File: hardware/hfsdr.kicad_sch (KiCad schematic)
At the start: 56 parts, among them J1 USB_C_Receptacle_USB2.0_16P, SW1 RST, SW2 BOOT0, SW4 EC12E2430803, U3 CH32V30xRxTx

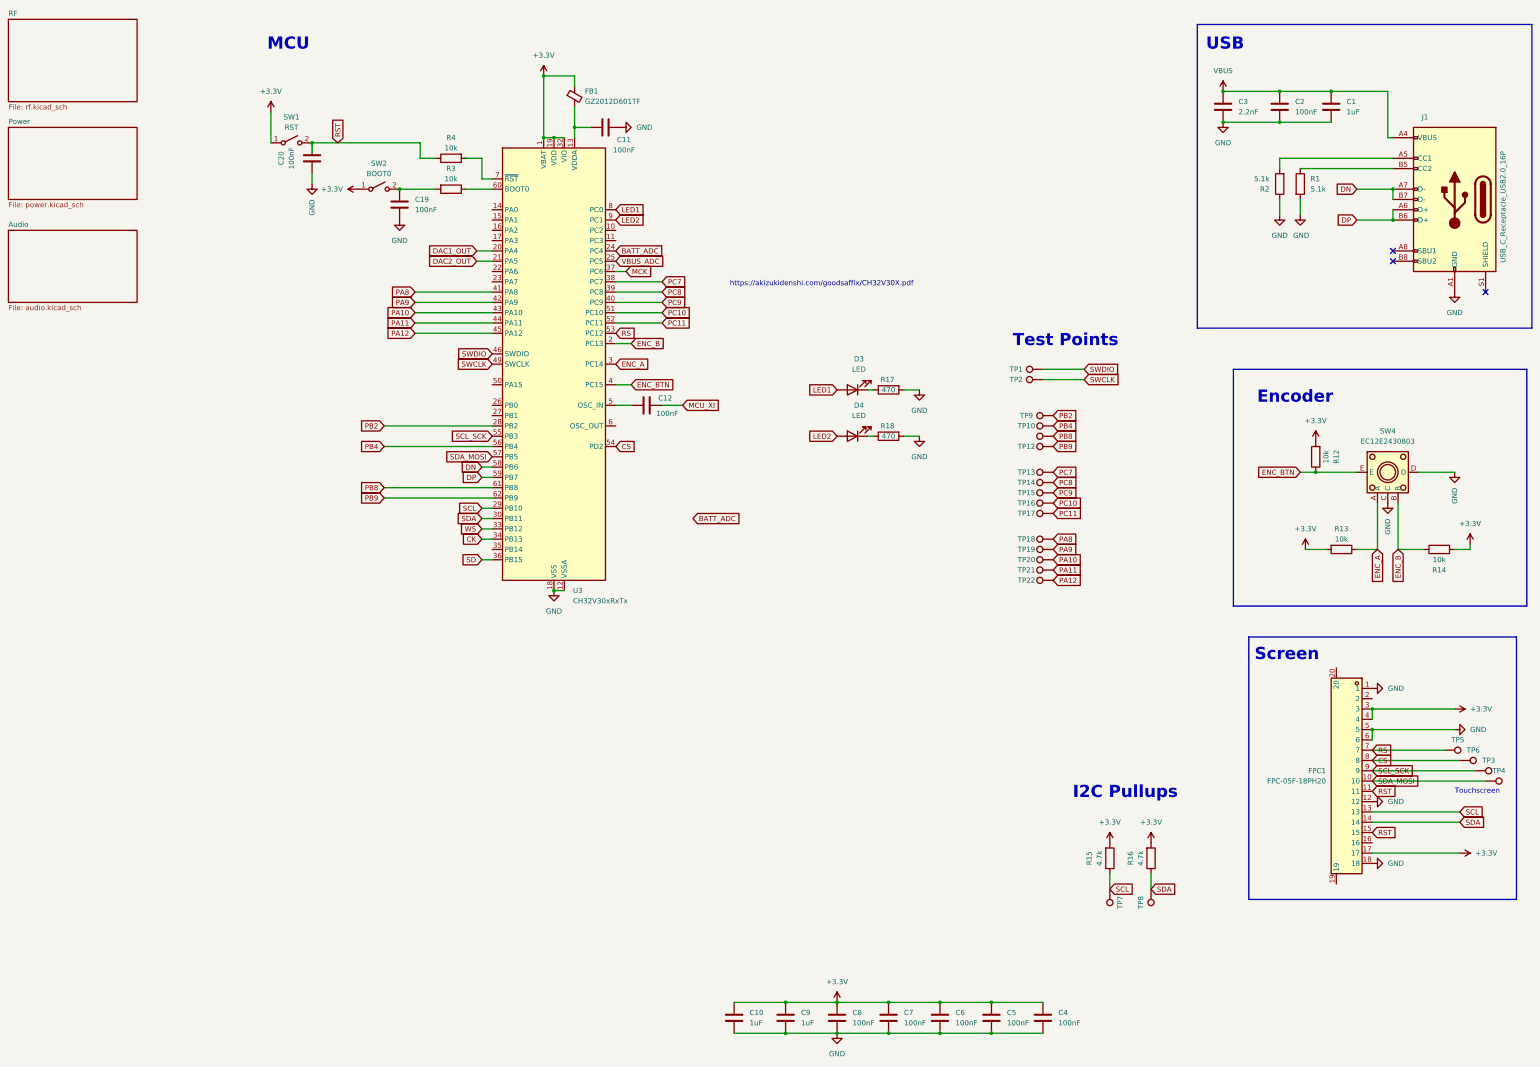
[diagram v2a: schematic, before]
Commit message: Update hardware
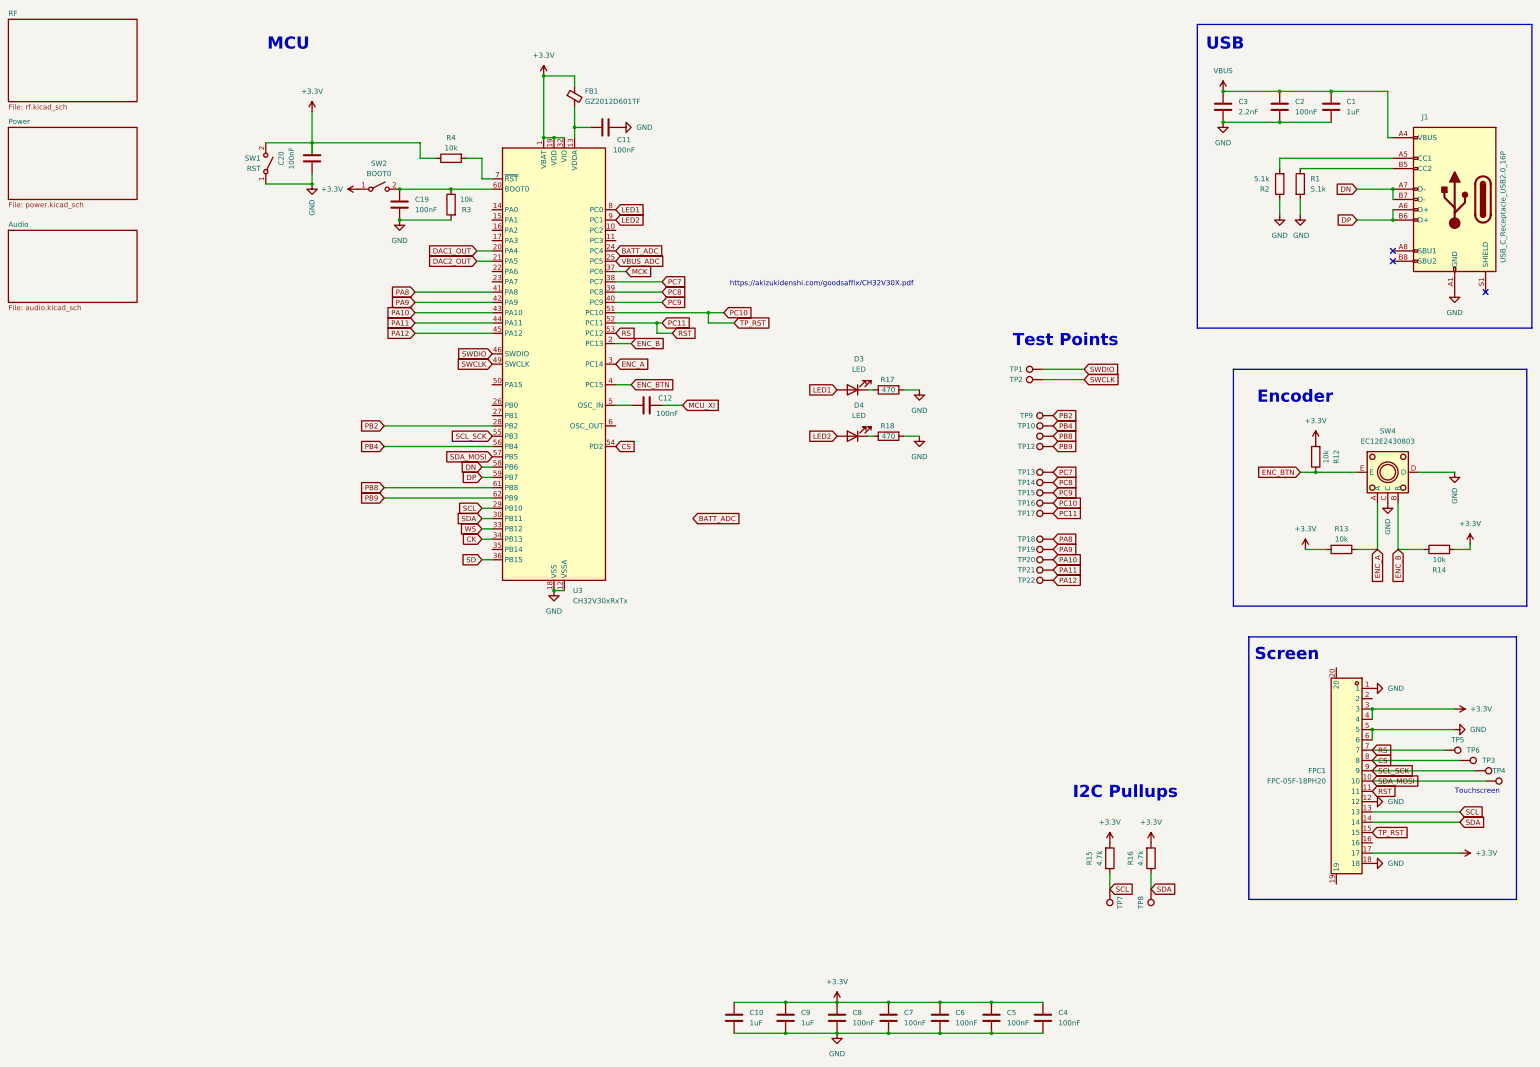
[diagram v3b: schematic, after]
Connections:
- net +3.3V: now also C20.2, R4.1, SW1.2 (B); no longer SW1.1 (A)
- net GND: now also R3.2, SW1.1 (A)
- net PC10: now also FPC1.15
- net PC11: now also FPC1.11
- net at C19.1, SW2.2 (B): now also R3.1, U3.60 (BOOT0); no longer R3.2
- removed net RST: C20.2, FPC1.11, FPC1.15, R4.1, SW1.2 (B)
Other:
- moved on the sheet: R3, SW1
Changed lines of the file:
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@@
 	)
 	(junction
+		(at 128.27 62.23)
+		(diameter 0)
+		(color 0 0 0 0)
+	)
+	(junction
+		(at 115.57 62.23)
+		(diameter 0)
+		(color 0 0 0 0)
+	)
+	(junction
 		(at 236.22 270.51)
 		(diameter 0)
@@
 	)
 	(junction
-		(at 115.57 62.23)
+		(at 93.98 60.96)
 		(diameter 0)
 		(color 0 0 0 0)
@@
 	)
 	(junction
+		(at 191.77 92.71)
+		(diameter 0)
+		(color 0 0 0 0)
+	)
+	(junction
+		(at 115.57 69.85)
+		(diameter 0)
+		(color 0 0 0 0)
+	)
+	(junction
 		(at 318.77 45.72)
 		(diameter 0)
@@
 	)
 	(junction
+		(at 179.07 95.25)
+		(diameter 0)
+		(color 0 0 0 0)
+	)
+	(junction
 		(at 360.68 62.23)
 		(diameter 0)
@@
 	(wire
 		(pts
-			(xy 83.82 43.18) (xy 83.82 50.8)
+			(xy 119.38 87.63) (xy 138.43 87.63)
 		)
 		(stroke
@@
 	(wire
 		(pts
-			(xy 119.38 87.63) (xy 138.43 87.63)
+			(xy 318.77 38.1) (xy 332.74 38.1)
 		)
 		(stroke
@@
 	(wire
 		(pts
-			(xy 318.77 38.1) (xy 332.74 38.1)
+			(xy 332.74 54.61) (xy 360.68 54.61)
 		)
 		(stroke
@@
 	(wire
 		(pts
-			(xy 332.74 54.61) (xy 360.68 54.61)
+			(xy 339.09 151.13) (xy 344.17 151.13)
 		)
 		(stroke
@@
 	(wire
 		(pts
-			(xy 339.09 151.13) (xy 344.17 151.13)
+			(xy 135.89 130.81) (xy 138.43 130.81)
 		)
 		(stroke
@@
 	(wire
 		(pts
-			(xy 135.89 130.81) (xy 138.43 130.81)
+			(xy 360.68 67.31) (xy 360.68 69.85)
 		)
 		(stroke
@@
 	(wire
 		(pts
-			(xy 360.68 67.31) (xy 360.68 69.85)
+			(xy 82.55 60.96) (xy 93.98 60.96)
 		)
 		(stroke
@@
 	(wire
 		(pts
-			(xy 115.57 62.23) (xy 124.46 62.23)
+			(xy 179.07 95.25) (xy 168.91 95.25)
 		)
 		(stroke
@@
 	(wire
 		(pts
+			(xy 198.12 95.25) (xy 191.77 95.25)
+		)
+		(stroke
+			(width 0)
+			(type default)
+		)
+	)
+	(wire
+		(pts
+			(xy 191.77 92.71) (xy 168.91 92.71)
+		)
+		(stroke
+			(width 0)
+			(type default)
+		)
+	)
+	(wire
+		(pts
 			(xy 248.92 270.51) (xy 261.62 270.51)
 		)
@@
 	(wire
 		(pts
+			(xy 93.98 43.18) (xy 93.98 50.8)
+		)
+		(stroke
+			(width 0)
+			(type default)
+		)
+	)
+	(wire
+		(pts
+			(xy 115.57 69.85) (xy 128.27 69.85)
+		)
+		(stroke
+			(width 0)
+			(type default)
+		)
+	)
+	(wire
+		(pts
 			(xy 377.19 203.2) (xy 355.6 203.2)
 		)
@@
 	(wire
 		(pts
-			(xy 180.34 92.71) (xy 168.91 92.71)
+			(xy 82.55 50.8) (xy 93.98 50.8)
+		)
+		(stroke
+			(width 0)
+			(type default)
+		)
+	)
+	(wire
+		(pts
+			(xy 195.58 92.71) (xy 191.77 92.71)
 		)
 		(stroke
@@
 	(wire
 		(pts
+			(xy 191.77 95.25) (xy 191.77 92.71)
+		)
+		(stroke
+			(width 0)
+			(type default)
+		)
+	)
+	(wire
+		(pts
 			(xy 180.34 115.57) (xy 185.42 115.57)
 		)
@@
 	(wire
 		(pts
+			(xy 115.57 62.23) (xy 128.27 62.23)
+		)
+		(stroke
+			(width 0)
+			(type default)
+		)
+	)
+	(wire
+		(pts
 			(xy 180.34 87.63) (xy 168.91 87.63)
 		)
@@
 	(wire
 		(pts
+			(xy 182.88 97.79) (xy 179.07 97.79)
+		)
+		(stroke
+			(width 0)
+			(type default)
+		)
+	)
+	(wire
+		(pts
 			(xy 381 205.74) (xy 355.6 205.74)
 		)
@@
 	(wire
 		(pts
-			(xy 180.34 95.25) (xy 168.91 95.25)
+			(xy 180.34 95.25) (xy 179.07 95.25)
 		)
 		(stroke
@@
 	(wire
 		(pts
+			(xy 179.07 97.79) (xy 179.07 95.25)
+		)
+		(stroke
+			(width 0)
+			(type default)
+		)
+	)
+	(wire
+		(pts
 			(xy 158.75 41.91) (xy 158.75 46.99)
 		)
@@
 	(wire
 		(pts
-			(xy 132.08 62.23) (xy 138.43 62.23)
+			(xy 128.27 62.23) (xy 138.43 62.23)
 		)
 		(stroke
@@
 		)
 	)
-	(global_label "RST"
-		(shape input)
-		(at 100.33 50.8 90)
-		(fields_autoplaced yes)
-		(effects
-			(font
-				(size 1.27 1.27)
-			)
-			(justify left)
-		)
-		(property "Intersheetrefs" "${INTERSHEET_REFS}"
-			(at 100.33 44.3677 90)
-			(effects
-				(font
-					(size 1.27 1.27)
-				)
-				(justify left)
-				(hide yes)
-			)
-		)
-	)
 	(global_label "PB8"
 		(shape input)
@@
 		)
 	)
+	(global_label "RST"
+		(shape input)
+		(at 182.88 97.79 0)
+		(fields_autoplaced yes)
+		(effects
+			(font
+				(size 1.27 1.27)
+			)
+			(justify left)
+		)
+		(property "Intersheetrefs" "${INTERSHEET_REFS}"
+			(at 189.3123 97.79 0)
+			(effects
+				(font
+					(size 1.27 1.27)
+				)
+				(justify left)
+				(hide yes)
+			)
+		)
+	)
+	(global_label "TP_RST"
+		(shape input)
+		(at 198.12 95.25 0)
+		(fields_autoplaced yes)
+		(effects
+			(font
+				(size 1.27 1.27)
+			)
+			(justify left)
+		)
+		(property "Intersheetrefs" "${INTERSHEET_REFS}"
+			(at 207.7575 95.25 0)
+			(effects
+				(font
+					(size 1.27 1.27)
+				)
+				(justify left)
+				(hide yes)
+			)
+		)
+	)
 	(global_label "VBUS_ADC"
 		(shape input)
@@
 		)
 	)
-	(global_label "RST"
+	(global_label "TP_RST"
 		(shape input)
 		(at 355.6 220.98 0)
@@
 		)
 		(property "Intersheetrefs" "${INTERSHEET_REFS}"
-			(at 362.0323 220.98 0)
+			(at 365.2375 220.98 0)
 			(effects
 				(font
@@
 	(global_label "PC10"
 		(shape input)
-		(at 180.34 92.71 0)
+		(at 195.58 92.71 0)
 		(fields_autoplaced yes)
 		(effects
@@
 		)
 		(property "Intersheetrefs" "${INTERSHEET_REFS}"
-			(at 188.2842 92.71 0)
+			(at 203.5242 92.71 0)
 			(effects
 				(font
@@
 	(symbol
 		(lib_id "power:+3.3V")
-		(at 83.82 43.18 0)
+		(at 93.98 43.18 0)
 		(unit 1)
 		(exclude_from_sim no)
@@
 		(fields_autoplaced yes)
 		(property "Reference" "#PWR025"
-			(at 83.82 46.99 0)
+			(at 93.98 46.99 0)
 			(effects
 				(font
@@
 		)
 		(property "Value" "+3.3V"
-			(at 83.82 38.1 0)
+			(at 93.98 38.1 0)
 			(effects
 				(font
@@
 		)
 		(property "Footprint" ""
-			(at 83.82 43.18 0)
+			(at 93.98 43.18 0)
 			(effects
 				(font
@@
 		)
 		(property "Datasheet" ""
-			(at 83.82 43.18 0)
+			(at 93.98 43.18 0)
 			(effects
 				(font
@@
 		)
 		(property "Description" "Power symbol creates a global label with name \"+3.3V\""
-			(at 83.82 43.18 0)
+			(at 93.98 43.18 0)
 			(effects
 				(font
@@
 	(symbol
 		(lib_id "Switch:SW_SPST")
-		(at 88.9 50.8 0)
+		(at 82.55 55.88 270)
+		(mirror x)
 		(unit 1)
 		(exclude_from_sim no)
@@
 		(on_board yes)
 		(dnp no)
-		(fields_autoplaced yes)
 		(property "Reference" "SW1"
-			(at 88.9 44.45 0)
+			(at 81.28 54.6099 90)
 			(effects
 				(font
 					(size 1.27 1.27)
 				)
+				(justify right)
 			)
 		)
 		(property "Value" "RST"
-			(at 88.9 46.99 0)
+			(at 81.28 57.1499 90)
 			(effects
 				(font
 					(size 1.27 1.27)
 				)
+				(justify right)
 			)
 		)
 		(property "Footprint" "Button_Switch_SMD:SW_Push_1P1T_XKB_TS-1187A"
-			(at 88.9 50.8 0)
+			(at 82.55 55.88 0)
 			(effects
 				(font
@@
 		)
 		(property "Datasheet" "~"
-			(at 88.9 50.8 0)
+			(at 82.55 55.88 0)
 			(effects
 				(font
@@
 		)
 		(property "Description" "Single Pole Single Throw (SPST) switch"
-			(at 88.9 50.8 0)
+			(at 82.55 55.88 0)
 			(effects
 				(font
@@
 	(symbol
 		(lib_id "Device:R")
-		(at 128.27 62.23 270)
+		(at 128.27 66.04 0)
+		(mirror y)
 		(unit 1)
 		(exclude_from_sim no)
@@
 		(dnp no)
 		(property "Reference" "R3"
-			(at 128.27 57.15 90)
+			(at 132.08 67.31 0)
 			(effects
 				(font
@@
 		)
 		(property "Value" "10k"
-			(at 128.27 59.69 90)
+			(at 132.08 64.77 0)
 			(effects
 				(font
@@
 		)
 		(property "Footprint" "Resistor_SMD:R_0805_2012Metric_Pad1.20x1.40mm_HandSolder"
-			(at 128.27 60.452 90)
+			(at 130.048 66.04 90)
 			(effects
 				(font
@@
 		)
 		(property "Datasheet" "~"
-			(at 128.27 62.23 0)
+			(at 128.27 66.04 0)
 			(effects
 				(font
@@
 		)
 		(property "Description" "Resistor"
-			(at 128.27 62.23 0)
+			(at 128.27 66.04 0)
 			(effects
 				(font
